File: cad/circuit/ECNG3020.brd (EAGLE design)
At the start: 84.8 x 61 mm, 22 parts, among them Q1 16Mhz, T1 2N3904, T2 2N3904, T3 2N3904, U1 ATMEGA328P-PU, X1 22-23-2021, X2 22-23-2021, X3 22-23-2021, X6 22-23-2021, X7 22-23-2021

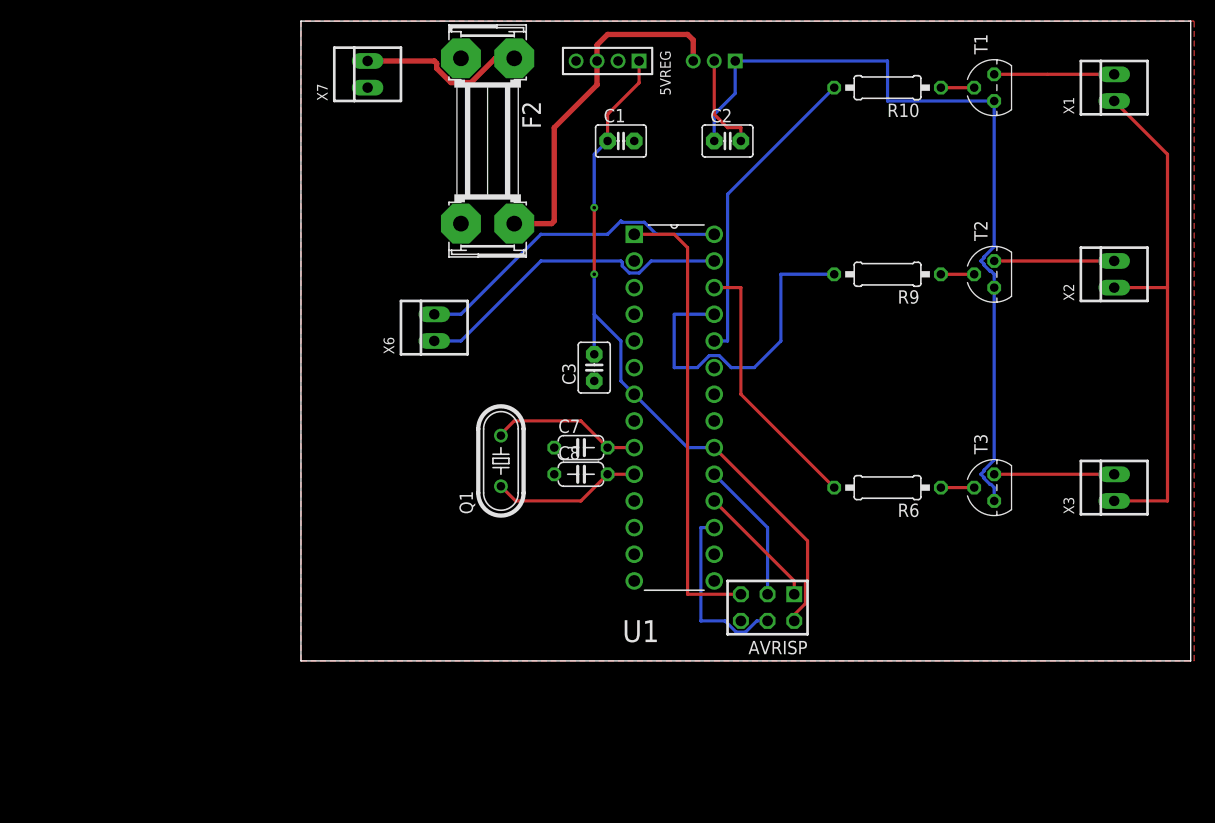
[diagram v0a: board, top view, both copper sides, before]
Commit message: Updated the schematic and board
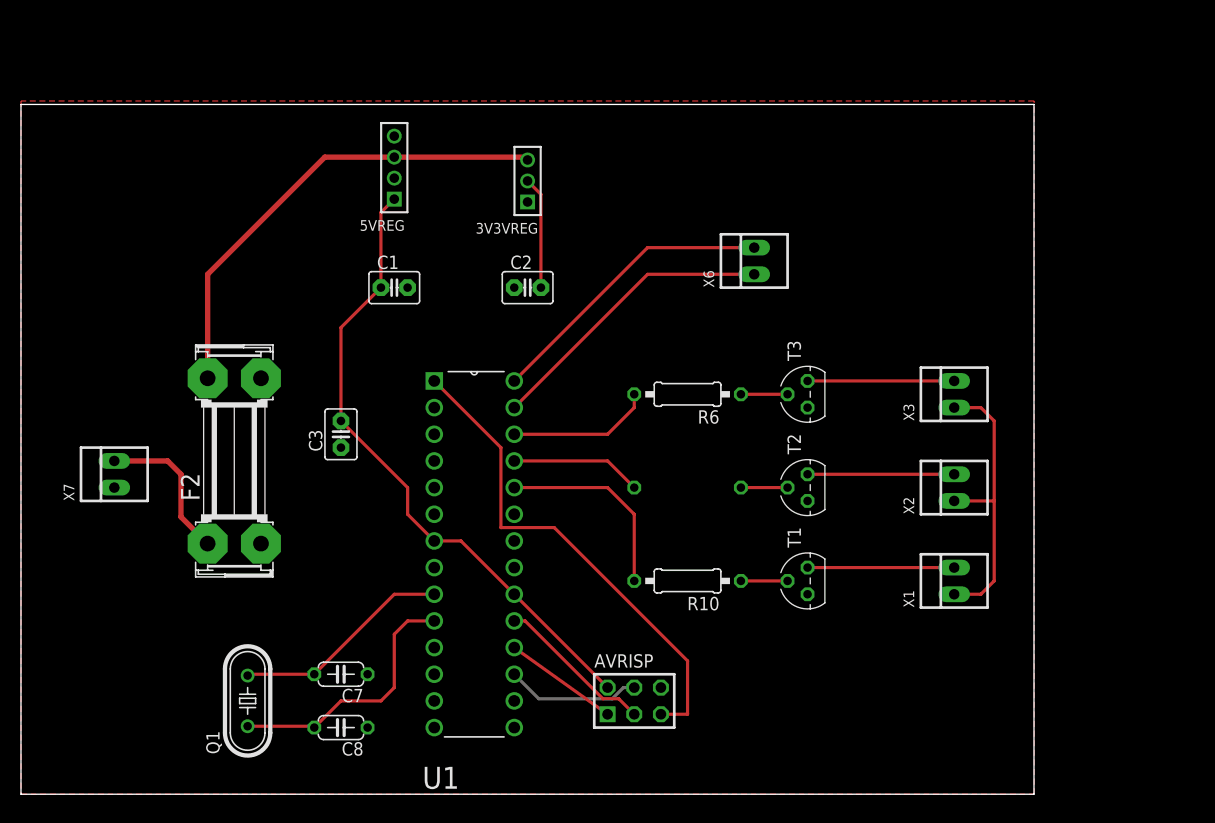
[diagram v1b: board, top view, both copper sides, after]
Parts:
- moved R10 50.7 mm to (63.5, 20.3)
- moved T1 50.2 mm to (74.9, 20.3)
- moved X1 49.4 mm to (88.9, 20.3)
- moved X7 45.1 mm to (8.89, 30.5)
- moved F2 38.9 mm to (20.3, 31.8), turned to 90 degrees
- moved C8 33.2 mm to (30.5, 6.35), turned to 180 degrees
- moved Q1 33.2 mm to (21.6, 8.89)
- moved C7 31.4 mm to (30.5, 11.4), turned to 180 degrees
- moved X6 31.1 mm to (69.8, 50.8)
- moved R9 27.9 mm to (63.5, 29.2), flipped to the bottom, turned to 0 degrees
- moved T2 27.0 mm to (74.9, 29.2)
- moved C1 25.7 mm to (35.6, 48.3)
- moved X2 25.4 mm to (88.9, 29.2)
- moved C3 25.0 mm to (30.5, 34.3)
- moved C2 23.6 mm to (48.3, 48.3)
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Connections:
- removed net RXM: U1.2
- removed net TXM: U1.3
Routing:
- net GND: track 77.2 -> 0.00 mm
- net N$7: track 50.4 -> 27.7 mm
- net N$2: track 32.5 -> 12.5 mm
- net N$4: track 25.3 -> 13.8 mm
- net 12V: track 34.2 -> 45.1 mm
- net N$1: track 29.6 -> 18.8 mm
- net N$5: track 14.3 -> 25.0 mm
- net VCC: track 69.3 -> 60.6 mm, vias 2 -> 0
- net N$3: track 14.4 -> 21.0 mm
- net MOSI: track 17.4 -> 12.8 mm
- net RST: track 43.7 -> 47.3 mm
- net SDA: track 31.0 -> 28.1 mm
- net SCL: track 30.9 -> 28.1 mm
- net N$12: track 11.4 -> 14.0 mm
- net N$11: track 11.4 -> 14.0 mm
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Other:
- board size 84.8 x 61 mm -> 96.5 x 65.7 mm
